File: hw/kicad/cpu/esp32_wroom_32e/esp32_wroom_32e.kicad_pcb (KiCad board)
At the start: 2 copper layers, 50 x 50 mm, 30 parts, among them J1 Conn_02x20_Odd_Even, J2 Conn_02x20_Odd_Even, U1 ESP32-WROOM-32, U2 ICM-42688-P

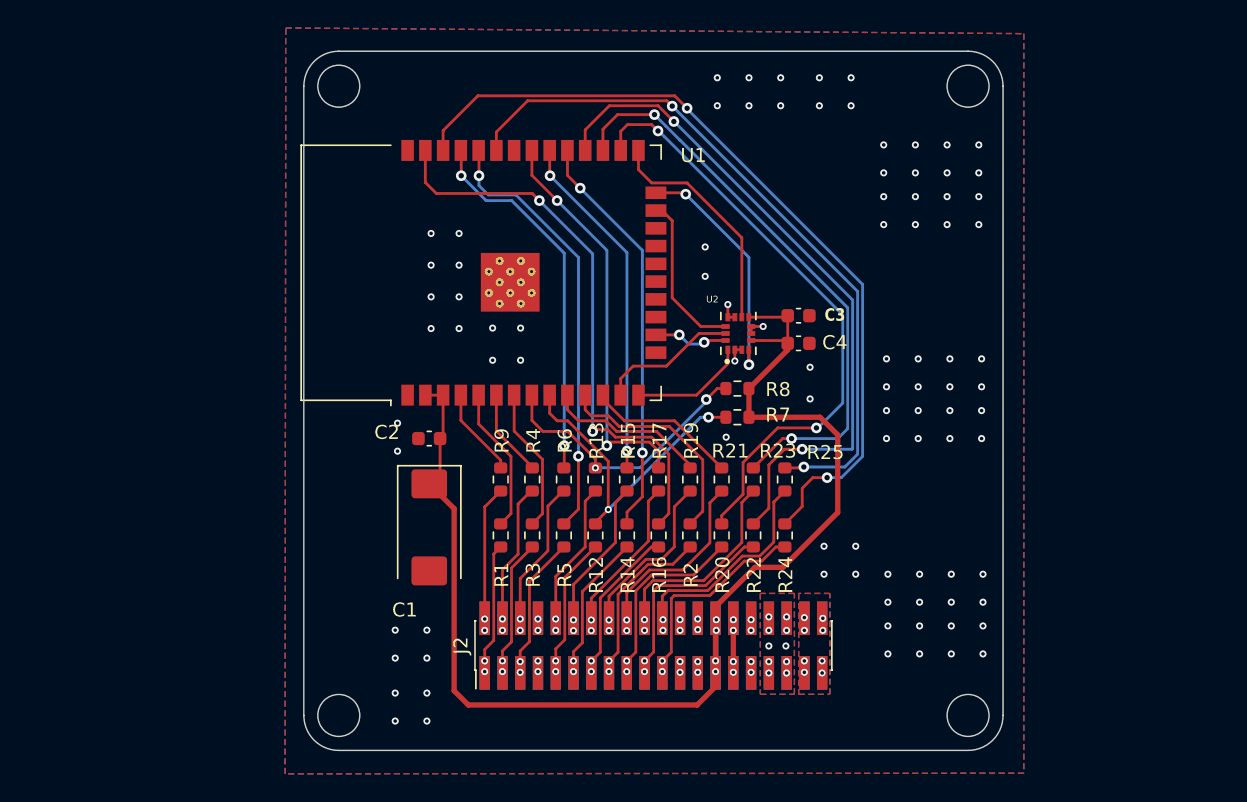
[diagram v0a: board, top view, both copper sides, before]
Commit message: 更新了template
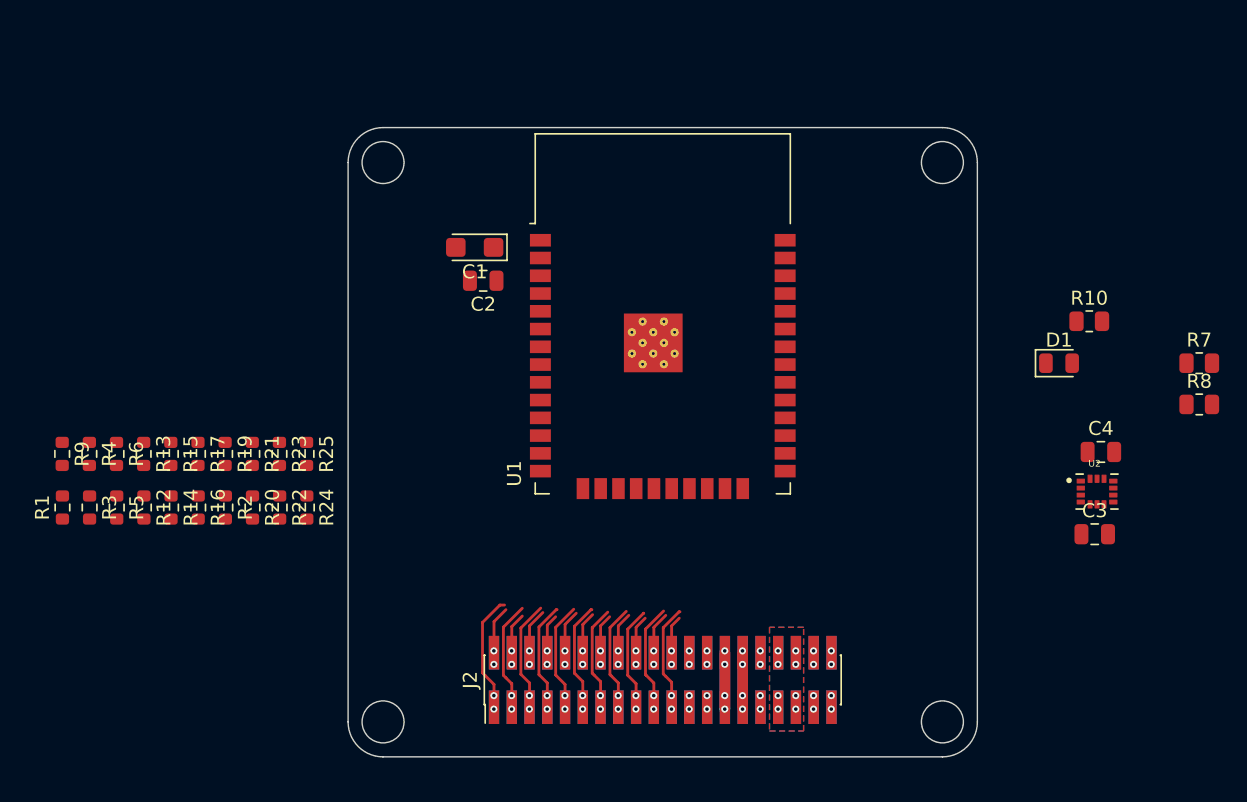
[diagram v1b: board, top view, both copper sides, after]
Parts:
- added D1: LED, LED_SMD:LED_0805_2012Metric, F.Cu at (104.7, 53.0)
- added R10: 10k, Resistor_SMD:R_0805_2012Metric, F.Cu at (106.9, 50.0)
- C1: value 200uF -> 47uF; footprint Capacitor_Tantalum_SMD:CP_EIA-7343-20_Kemet-V -> Capacitor_Tantalum_SMD:CP_EIA-3216-12_Kemet-S
- C2, C3, C4: footprint Capacitor_SMD:C_0603_1608Metric -> Capacitor_SMD:C_0805_2012Metric
- R7, R8: footprint Resistor_SMD:R_0603_1608Metric -> Resistor_SMD:R_0805_2012Metric
- moved R25 34.3 mm to (50.9, 59.5)
- moved R24 34.2 mm to (50.9, 63.4)
- moved R23 33.9 mm to (49.0, 59.5)
- moved R22 33.9 mm to (49.0, 63.4)
- moved R21 33.6 mm to (47.0, 59.5)
- moved R20 33.6 mm to (47.0, 63.4)
- moved R19 33.3 mm to (45.1, 59.5)
- moved R2 33.3 mm to (45.1, 63.4)
- moved R7 33.3 mm to (114.8, 53.0), turned to 0 degrees
- moved R8 33.0 mm to (114.8, 56.0), turned to 0 degrees
- moved R17 33.0 mm to (43.1, 59.5)
- moved R16 33.0 mm to (43.2, 63.4)
- moved R15 32.7 mm to (41.2, 59.5)
- moved R14 32.7 mm to (41.2, 63.4)
- moved R13 32.4 mm to (39.3, 59.5)
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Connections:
- U1 pad 24: /IMU_INT1 -> /LED
- U2 pad 4: /IMU_INT1 -> unconnected-(U2-INT1/INT-Pad4)
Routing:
- net +3.3V: track 90.7 -> 7.94 mm
- net /pwm7: track 58.7 -> 0.00 mm, vias 2 -> 0
- net /pwm8: track 51.0 -> 0.00 mm, vias 2 -> 0
- net /pwm5: track 48.8 -> 0.00 mm, vias 2 -> 0
- net /pwm3: track 43.3 -> 0.00 mm, vias 2 -> 0
- net /pwm6: track 41.7 -> 0.00 mm, vias 2 -> 0
- net /vspi_mosi: track 40.6 -> 0.00 mm, vias 2 -> 0
- net /uart0rx: track 31.3 -> 0.00 mm, vias 2 -> 0
- net /vspi_cs: track 29.4 -> 0.00 mm, vias 2 -> 0
- net /vspi_miso: track 28.6 -> 0.00 mm, vias 2 -> 0
- net /uart0tx: track 26.8 -> 0.00 mm, vias 2 -> 0
- net /vspi1_clk: track 25.0 -> 0.00 mm, vias 2 -> 0
- net /i2c_data: track 23.0 -> 0.00 mm, vias 2 -> 0
- net /i2c_clock: track 19.9 -> 0.00 mm, vias 2 -> 0
- net /IMU_INT1: track 17.3 -> 0.00 mm, vias 2 -> 0
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- removed copper zone on B.Cu, net GND
- removed copper zone on F.Cu, net GND
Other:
- board size 50 x 50 mm -> 45 x 45 mm
